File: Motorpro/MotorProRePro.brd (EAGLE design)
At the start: 100 x 80 mm, 19 parts, among them IC1 7805T, Q1 BTA06-600BRG

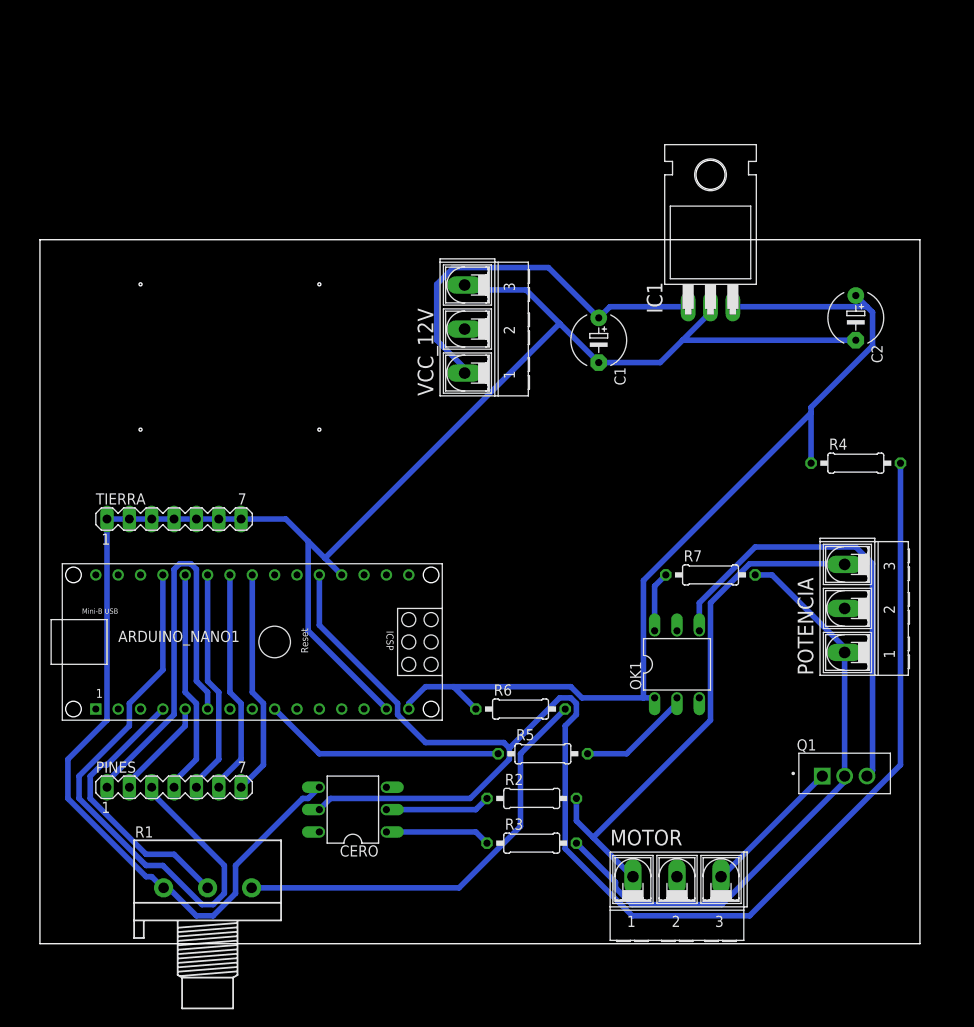
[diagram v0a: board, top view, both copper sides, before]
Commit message: Board modificada
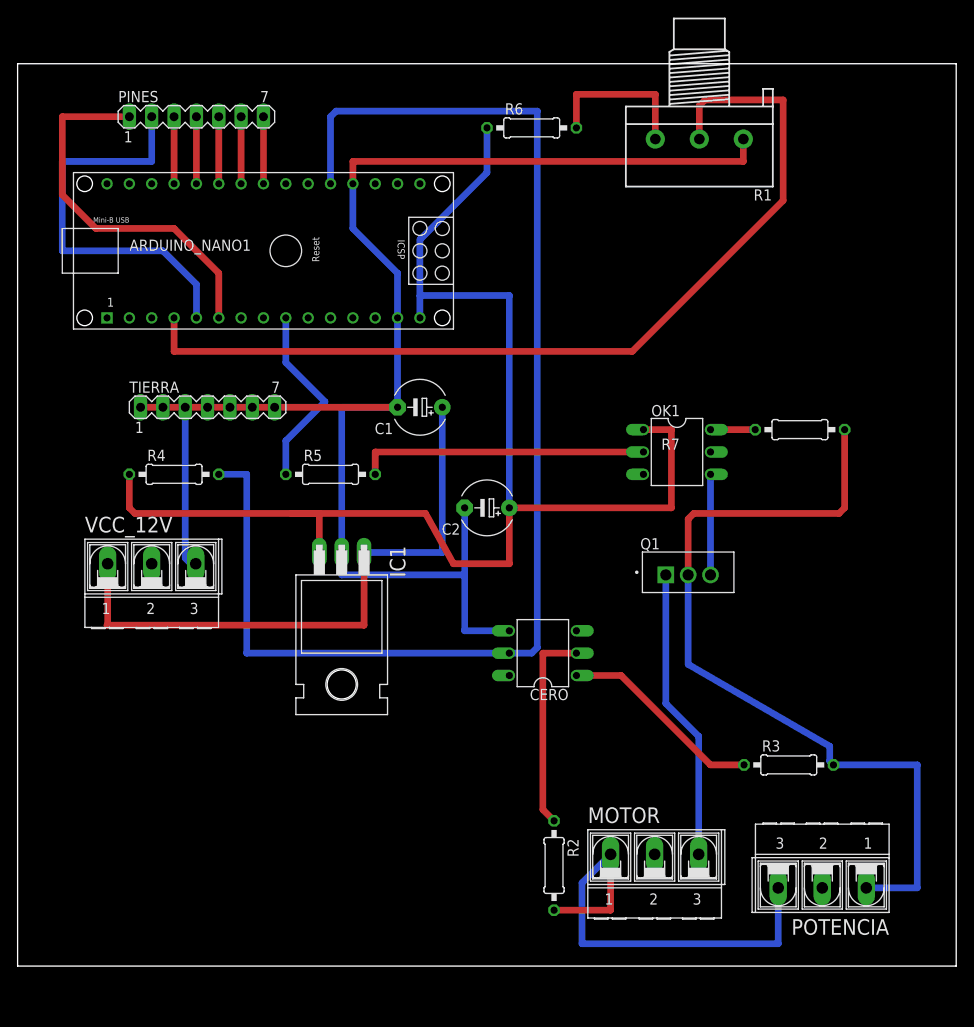
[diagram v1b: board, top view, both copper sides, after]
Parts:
- moved R1 101.8 mm to (74.9, 91.4), turned to 180 degrees
- moved R4 77.5 mm to (15.2, 53.3)
- moved PINES 76.2 mm to (17.8, 94.0)
- moved R6 66.1 mm to (55.9, 92.7)
- moved IC1 63.9 mm to (34.3, 34.3), turned to 180 degrees
- moved C2 47.1 mm to (50.8, 49.5), turned to 180 degrees
- moved ARDUINO_NANO1 44.5 mm to (27.9, 78.7)
- moved VCC_12V 44.4 mm to (12.7, 43.2), turned to 0 degrees
- moved R5 39.9 mm to (33.0, 53.3)
- moved POTENCIA 31.9 mm to (88.9, 6.35), turned to 180 degrees
- moved R3 30.5 mm to (85.1, 20.3)
- moved Q1 29.0 mm to (71.1, 41.9)
- moved CERO 28.0 mm to (57.1, 33.0)
- moved OK1 24.1 mm to (72.4, 55.9), turned to 270 degrees
- moved C1 21.7 mm to (43.2, 61.0), turned to 180 degrees
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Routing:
- net REFERENCIA: track 31.5 -> 105.2 mm
- net N$13: track 66.9 -> 7.62 mm
- net VCC: track 111.7 -> 154.1 mm
- net N$8: track 50.7 -> 11.4 mm
- net GND: track 220.0 -> 183.2 mm
- net N$14: track 11.5 -> 46.0 mm
- net N$5: track 48.9 -> 17.9 mm
- net N$1: track 43.7 -> 69.9 mm
- net FASE: track 68.4 -> 93.9 mm
- net ZERO: track 169.0 -> 149.1 mm
- net N$4: track 13.2 -> 33.0 mm
- net N$9: track 25.7 -> 7.62 mm
- net N$12: track 25.7 -> 7.62 mm
- net N$11: track 25.7 -> 7.62 mm
- net N$10: track 25.7 -> 7.62 mm
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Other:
- board size 100 x 80 mm -> 106.7 x 102.5 mm
